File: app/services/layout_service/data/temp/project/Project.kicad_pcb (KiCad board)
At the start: 2 copper layers, 40 x 40 mm, 58 parts

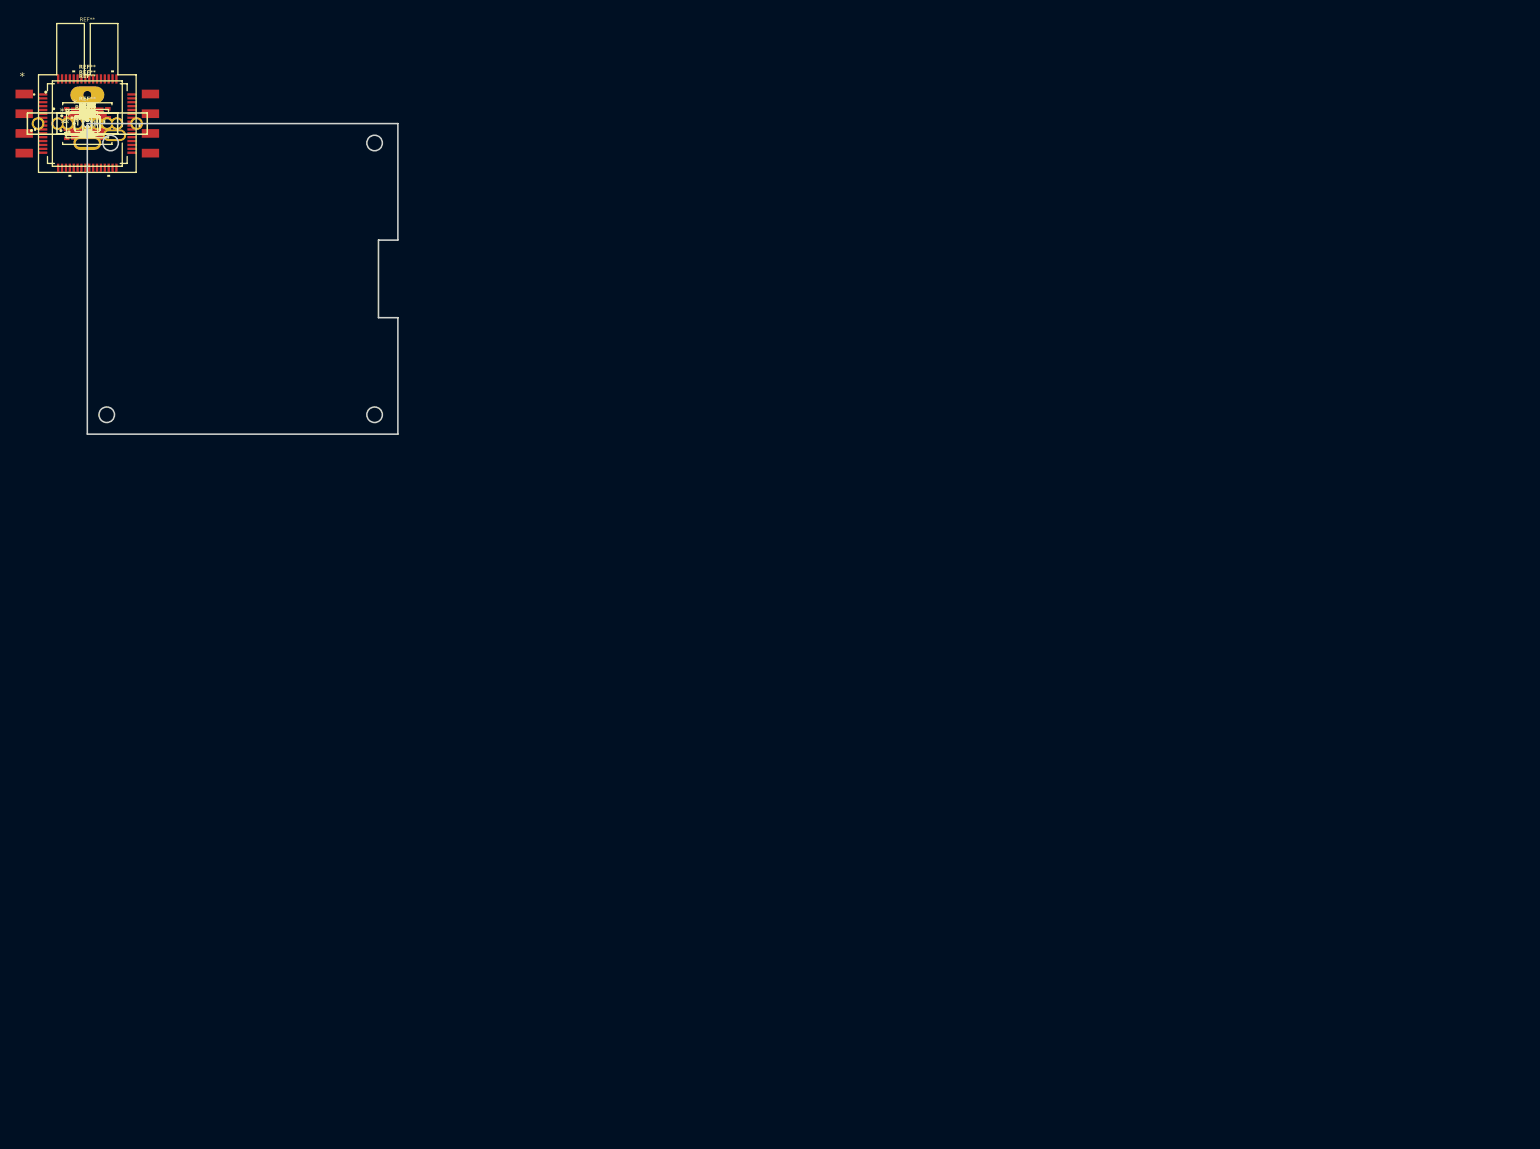
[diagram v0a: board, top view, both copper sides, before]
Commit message: 流程适配-开始考虑焊盘和旋转
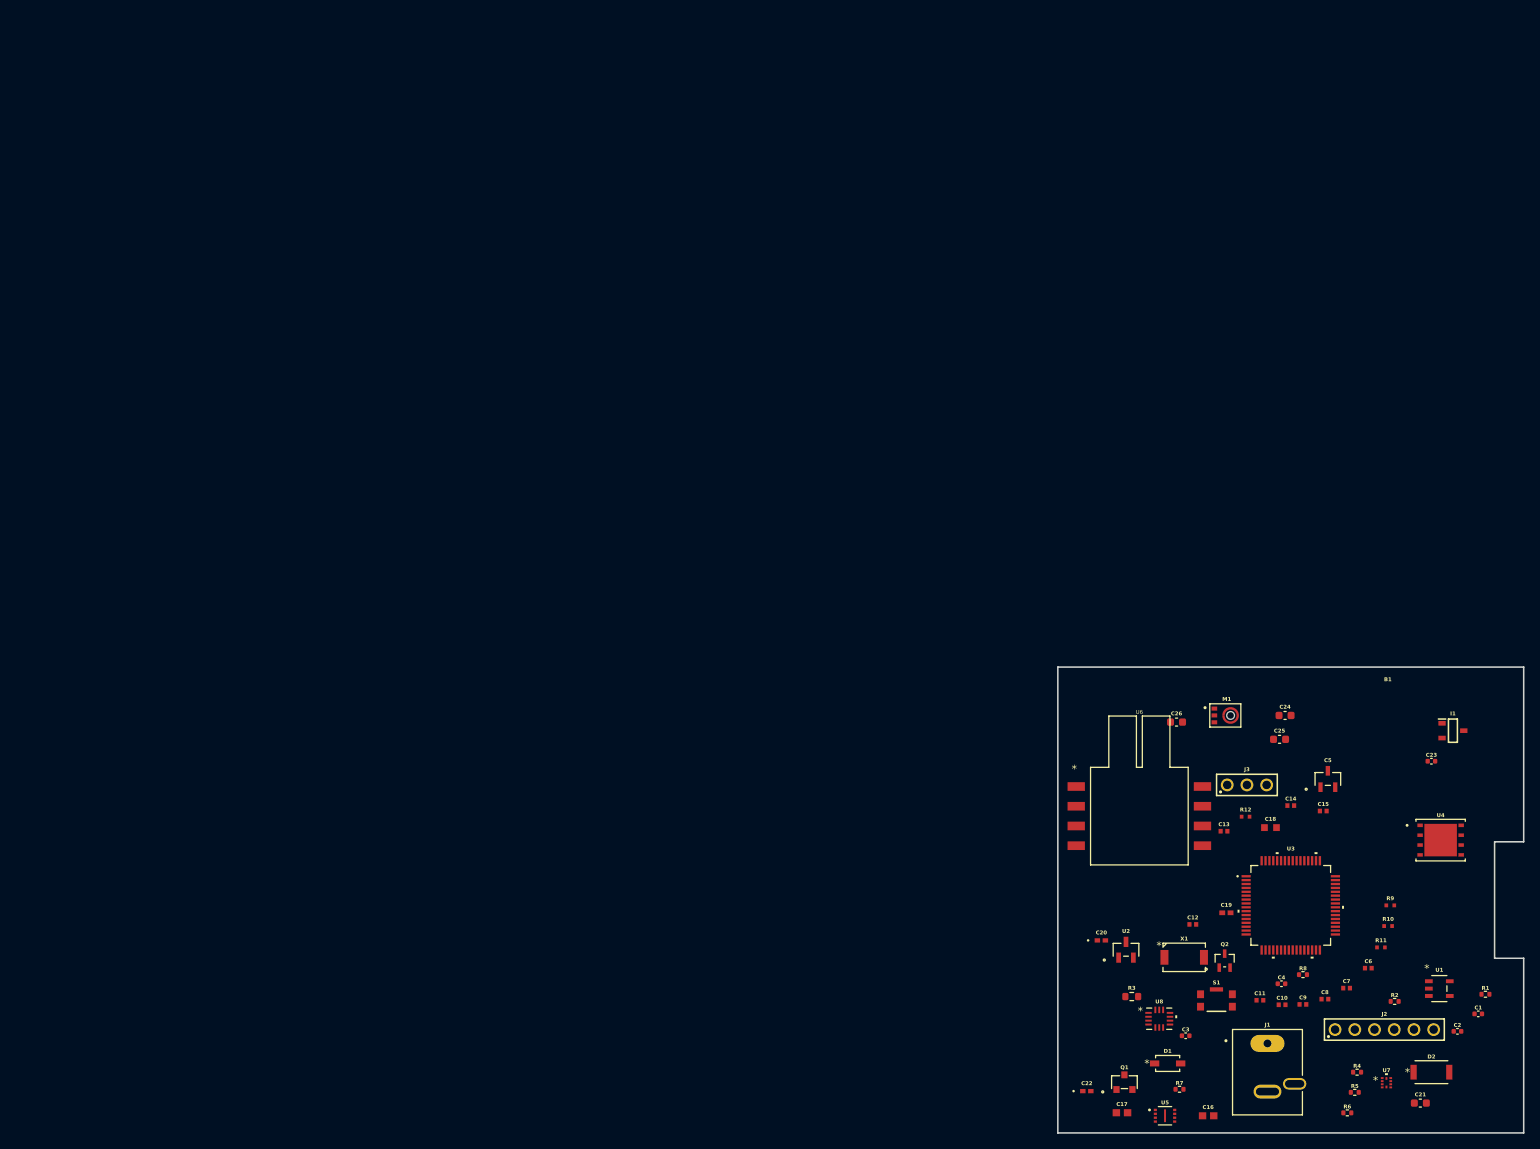
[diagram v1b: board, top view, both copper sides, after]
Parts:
- removed IC**: SOT95P285X113-3N, SOT95P285X113-3N
- removed REF** (x4): C_0603_1608Metric, C_0603_1608Metric
- removed REF**: 8L_USON_2X3_ISI, 8L_USON_2X3_ISI
- removed REF** (x2): YAG_CC0603_YAG, YAG_CC0603_YAG
- removed REF** (x2): CAP_0402_SAM, CAP_0402_SAM
- removed REF**: BMX160_BOS, BMX160_BOS
- removed REF**: SOT23-3_LTF, SOT23-3_LTF
- removed REF** (x7): R_0402_1005Metric, R_0402_1005Metric
- removed REF** (x5): C_0402_1005Metric, C_0402_1005Metric
- removed REF**: MC3635_MEM, MC3635_MEM
- removed REF**: SOT25_DIO, SOT25_DIO
- removed REF**: SOD-123_ONS, SOD-123_ONS
- removed REF**: CUI_PJ-044A, CUI_PJ-044A
- removed REF**: SDO_CFP5_SOD128_NEX, SDO_CFP5_SOD128_NEX
- removed REF**: CAP_CL10A105KB8NNN_SAM, CAP_CL10A105KB8NNN_SAM
- removed REF**: SOT-23_DIO, SOT-23_DIO
- removed REF**: SOT-323_DIO, SOT-323_DIO
- removed REF**: R_0603_1608Metric, R_0603_1608Metric
- removed REF**: SOT-23_MC_MCH, SOT-23_MC_MCH
- removed REF**: Battery_CR1225, Battery_CR1225
- removed REF**: MR25H40CDC_EVS, MR25H40CDC_EVS
- removed REF**: LQFP64-10x10mm, STM32F103RET6
- removed REF**: 1351-01_NXP, 1351-01_NXP
- removed REF** (x4): RES_ERJ-2GEJ103X, 0402R
- removed REF**: 61300611121, 61300611121
- removed REF** (x10): CAPC1005X55N, 0402C
- removed REF**: SW_KMR221GLFS, KMR221GLFS
- removed REF**: 0402_AVX, 0402_AVX
- removed REF**: XTAL_NX5032GA-16.000M-STD-CSU-2_NDK, NX5032GA_16_000M_STD_CSU_2
- removed REF**: 61300311121, 61300311121
- removed REF**: MIC_ICS-40720, MIC_ICS-40720
- added B1: Battery_CR1225, Battery_CR1225, F.Cu at (167.5, 78.2)
- added C1: C_0402_1005Metric, C_0402_1005Metric, F.Cu at (179.1, 114.7)
- added C10: CAPC1005X55N, 0402C, F.Cu at (153.9, 113.5)
- added C11: CAPC1005X55N, 0402C, F.Cu at (151.0, 112.9)
- added C12: CAPC1005X55N, 0402C, F.Cu at (142.4, 103.1)
- added C13: CAPC1005X55N, 0402C, F.Cu at (146.4, 91.1)
- added C14: CAPC1005X55N, 0402C, F.Cu at (155.0, 87.8)
- added C15: CAPC1005X55N, 0402C, F.Cu at (159.2, 88.5)
- added C16: YAG_CC0603_YAG, YAG_CC0603_YAG, F.Cu at (144.4, 127.8)
- added C17: YAG_CC0603_YAG, YAG_CC0603_YAG, F.Cu at (133.3, 127.4)
- added C18: CAP_CL10A105KB8NNN_SAM, CAP_CL10A105KB8NNN_SAM, F.Cu at (152.4, 90.7)
- added C19: 0402_AVX, 0402_AVX, F.Cu at (146.7, 101.6)
- added C2: C_0402_1005Metric, C_0402_1005Metric, F.Cu at (176.5, 116.9)
- added C20: CAP_0402_SAM, CAP_0402_SAM, F.Cu at (130.6, 105.2)
- added C21: C_0603_1608Metric, C_0603_1608Metric, F.Cu at (171.7, 126.2)
- added C22: CAP_0402_SAM, CAP_0402_SAM, F.Cu at (128.7, 124.6)
- added C23: C_0402_1005Metric, C_0402_1005Metric, F.Cu at (173.1, 82.1)
- added C24: C_0603_1608Metric, C_0603_1608Metric, F.Cu at (154.3, 76.2)
- added C25: C_0603_1608Metric, C_0603_1608Metric, F.Cu at (153.6, 79.3)
- added C26: C_0603_1608Metric, C_0603_1608Metric, F.Cu at (140.3, 77.1)
- added C3: C_0402_1005Metric, C_0402_1005Metric, F.Cu at (141.5, 117.5)
- added C4: C_0402_1005Metric, C_0402_1005Metric, F.Cu at (153.8, 110.8)
- added C5: SOT23-3_LTF, SOT23-3_LTF, F.Cu at (159.8, 84.4)
- added C6: CAPC1005X55N, 0402C, F.Cu at (165.0, 108.8)
- added C7: CAPC1005X55N, 0402C, F.Cu at (162.2, 111.3)
- added C8: CAPC1005X55N, 0402C, F.Cu at (159.4, 112.8)
- added C9: CAPC1005X55N, 0402C, F.Cu at (156.6, 113.4)
- added D1: SOD-123_ONS, SOD-123_ONS, F.Cu at (139.1, 121.1)
- added D2: SDO_CFP5_SOD128_NEX, SDO_CFP5_SOD128_NEX, F.Cu at (173.1, 122.2)
- added I1: SOT95P285X113-3N, SOT95P285X113-3N, F.Cu at (175.9, 78.2)
- added J1: CUI_PJ-044A, CUI_PJ-044A, F.Cu at (152.0, 122.2)
- added J2: 61300611121, 61300611121, F.Cu at (167.1, 116.7)
- added J3: 61300311121, 61300311121, F.Cu at (149.4, 85.2)
- added M1: MIC_ICS-40720, MIC_ICS-40720, F.Cu at (147.2, 76.2)
- added Q1: SOT-23_DIO, SOT-23_DIO, F.Cu at (133.6, 123.5)
- added Q2: SOT-323_DIO, SOT-323_DIO, F.Cu at (146.5, 107.8)
- added R1: R_0402_1005Metric, R_0402_1005Metric, F.Cu at (180.1, 112.1)
- added R10: RES_ERJ-2GEJ103X, 0402R, F.Cu at (167.5, 103.4)
- added R11: RES_ERJ-2GEJ103X, 0402R, F.Cu at (166.6, 106.1)
- added R12: RES_ERJ-2GEJ103X, 0402R, F.Cu at (149.2, 89.3)
- added R2: R_0402_1005Metric, R_0402_1005Metric, F.Cu at (168.4, 113.1)
- added R3: R_0603_1608Metric, R_0603_1608Metric, F.Cu at (134.5, 112.4)
- added R4: R_0402_1005Metric, R_0402_1005Metric, F.Cu at (163.5, 122.2)
- added R5: R_0402_1005Metric, R_0402_1005Metric, F.Cu at (163.2, 124.8)
- added R6: R_0402_1005Metric, R_0402_1005Metric, F.Cu at (162.3, 127.4)
- added R7: R_0402_1005Metric, R_0402_1005Metric, F.Cu at (140.7, 124.4)
- added R8: R_0402_1005Metric, R_0402_1005Metric, F.Cu at (156.6, 109.6)
- added R9: RES_ERJ-2GEJ103X, 0402R, F.Cu at (167.8, 100.7)
- added S1: SW_KMR221GLFS, KMR221GLFS, F.Cu at (145.4, 112.9)
- added U1: SOT25_DIO, SOT25_DIO, F.Cu at (174.1, 111.4)
- added U2: SOT-23_MC_MCH, SOT-23_MC_MCH, F.Cu at (133.8, 106.4)
- added U3: LQFP64-10x10mm, STM32F103RET6, F.Cu at (155.0, 100.7)
- added U4: MR25H40CDC_EVS, MR25H40CDC_EVS, F.Cu at (174.3, 92.3)
- added U5: 8L_USON_2X3_ISI, 8L_USON_2X3_ISI, F.Cu at (138.8, 127.8)
- added U6: 1351-01_NXP, 1351-01_NXP, F.Cu at (135.5, 89.2)
- added U7: MC3635_MEM, MC3635_MEM, F.Cu at (167.3, 123.5)
- added U8: BMX160_BOS, BMX160_BOS, F.Cu at (138.1, 115.3)
- added X1: XTAL_NX5032GA-16.000M-STD-CSU-2_NDK, NX5032GA_16_000M_STD_CSU_2, F.Cu at (141.3, 107.4)
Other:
- board size 40 x 40 mm -> 60 x 60 mm
